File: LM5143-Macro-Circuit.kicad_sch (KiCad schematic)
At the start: 54 parts, among them Q2 NTMFS4D0N08XT1G, U10 NTMFS4D0N08XT1G, U11 NTMFS4D0N08XT1G, U14 NTMFS4D0N08XT1G, U15 NTMFS4D0N08XT1G, U8 LM5145

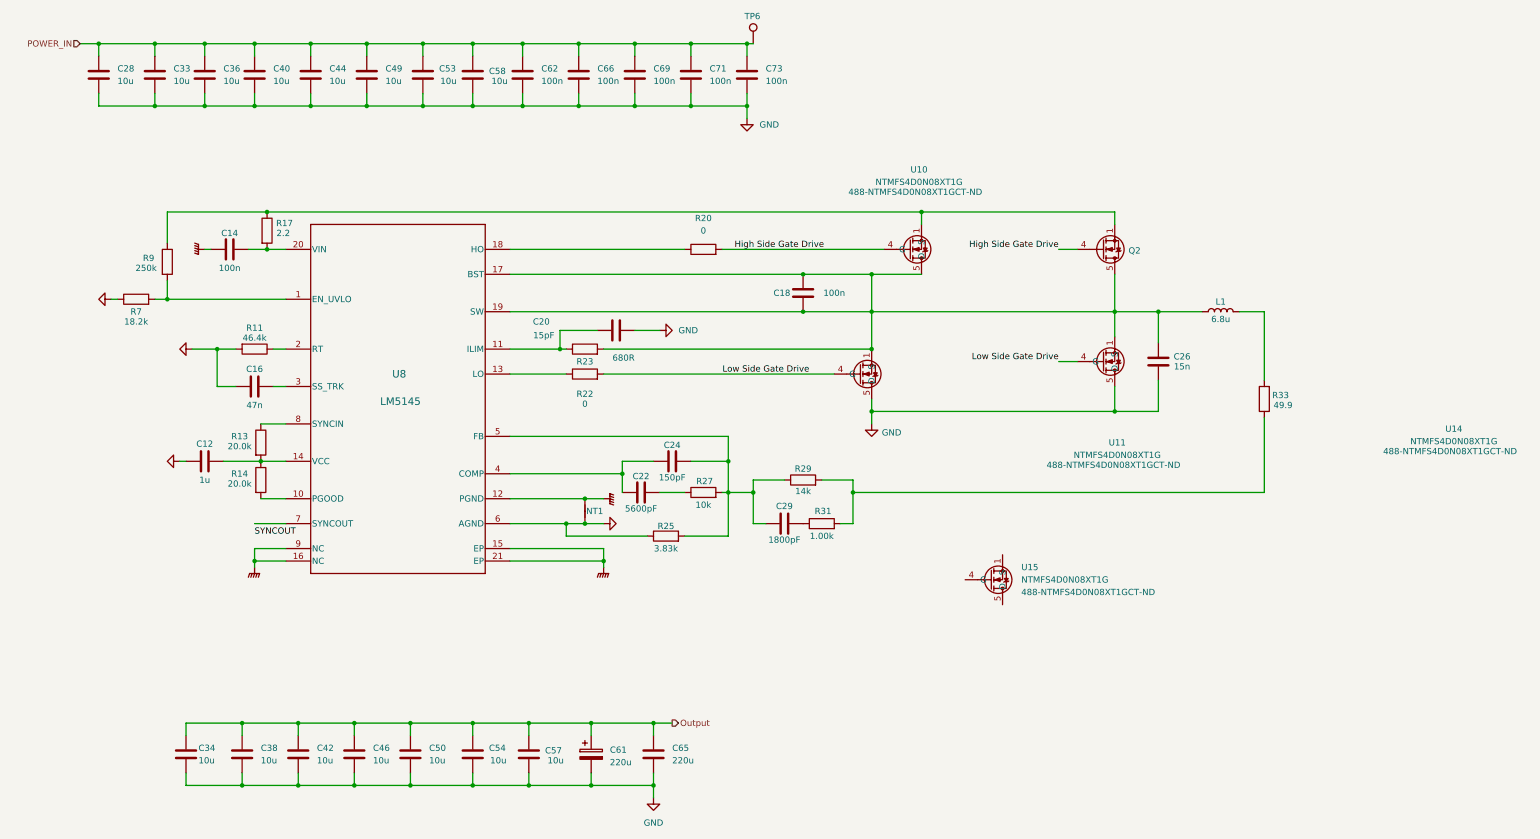
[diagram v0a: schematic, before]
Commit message: Started Layout and cleaned up schematic
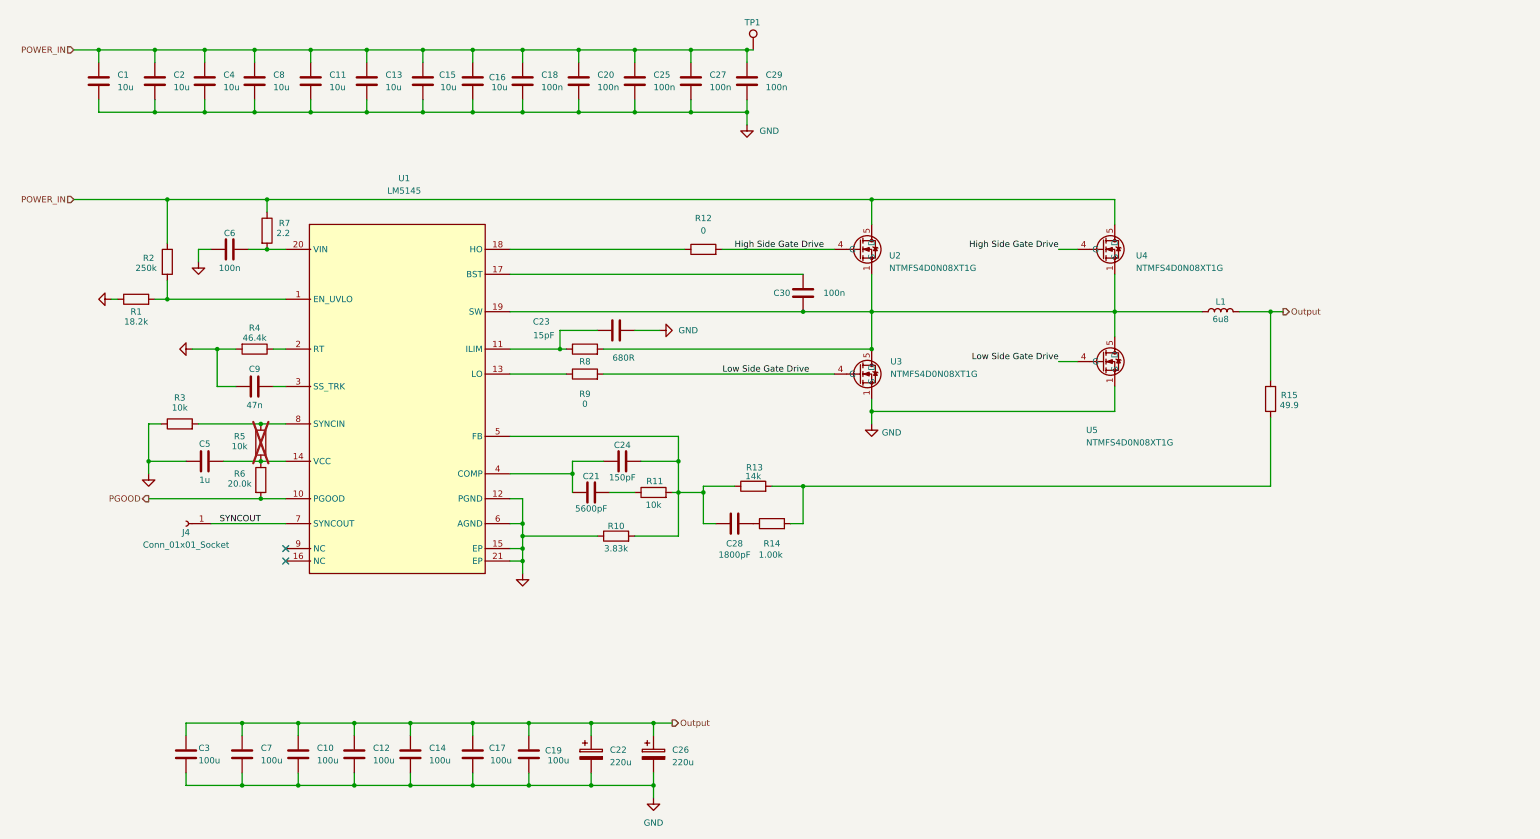
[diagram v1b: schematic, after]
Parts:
- removed C26: 15n, Capacitor_SMD:C_0603_1608Metric, symbol Device:C
- removed C65: 220u, Capacitor_SMD:C_0603_1608Metric, symbol Device:C
- removed NT1: NetTie_2, NetTie:NetTie-2_SMD_Pad0.5mm, symbol Device:NetTie_2
- removed Q2: NTMFS4D0N08XT1G, ecocad_lib_footprints:PowerMosDFNHybrid, symbol Transistor_FET:CSD18563Q5A
- removed U10, U11, U14, U15: NTMFS4D0N08XT1G, ecocad_lib_footprints:PowerMosDFNHybrid, symbol ecocad_lib_symbols:NTMFS4D0N08XT1G
- removed U8: LM5145, ecocad_lib_footprints:RGY0024F-MFG, symbol 2024-07-27_02-47-30:LM5145RGYR
- added C26: 220u, ecocad_lib_footprints:CAP_EEE1HA221P, symbol Device:C_Polarized
- added J4: Conn_01x01_Socket, Connector_PinHeader_2.54mm:PinHeader_1x01_P2.54mm_Vertical, symbol Connector:Conn_01x01_Socket
- added R3: 10k, Resistor_SMD:R_0603_1608Metric, symbol Device:R
- added U1: LM5145, Texas_RGY_R-PVQFN-N20_EP2.05x3.05mm_ThermalVias, symbol ecocad_lib_symbols:LM5145
- added U2, U3, U4, U5: NTMFS4D0N08XT1G, ecocad_lib_footprints:PowerMosDFNHybrid, symbol ecocad_lib_symbols:NTMFS4D0N08XT1G
- C10: renamed from C42; value 10u -> 100u
- C12: renamed from C46; value 10u -> 100u
- C14: renamed from C50; value 10u -> 100u
- C17: renamed from C54; value 10u -> 100u
- C19: renamed from C57; value 10u -> 100u
- C22: renamed from C61; footprint Capacitor_SMD:C_0603_1608Metric -> ecocad_lib_footprints:CAP_EEE1HA221P
- C3: renamed from C34; value 10u -> 100u
- C7: renamed from C38; value 10u -> 100u
- L1: value 6.8u -> 6u8
- R5: renamed from R13; value 20.0k -> 10k; now not fitted
- renumbered C28 to C1, C44 to C11, C49 to C13, C53 to C15, C58 to C16, C62 to C18, C33 to C2, C66 to C20, C22 to C21, C20 to C23, C69 to C25, C71 to C27, C29 to C28, C73 to C29, C18 to C30, C36 to C4, C12 to C5, C14 to C6, C40 to C8, C16 to C9, R7 to R1, R25 to R10, R27 to R11, R20 to R12, R29 to R13, R31 to R14, R33 to R15, R9 to R2, R11 to R4, R14 to R6, R17 to R7, R23 to R8, R22 to R9, TP6 to TP1
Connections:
- net GNDPWR is gone; now on net GND: C6.1
- net GND: now also C26.2, R3.1, U1.12 (PGND), U1.15 (EP), U1.21 (EP), U1.6 (AGND), U3.1 (S), U3.2 (S), U3.3 (S), U5.1 (S), U5.2 (S), U5.3 (S)
- net High Side Gate Drive: now also U2.4 (G), U4.4 (G)
- net Low Side Gate Drive: now also U3.4 (G), U5.4 (G)
- net Output: now also L1.2, R15.2, C26.1
- net POWER_IN: now also R2.1, R7.1, U2.5 (D), U4.5 (D)
- net SYNCOUT: now also J4.1 (Pin_1), U1.7 (SYNCOUT)
- net at C30.1, L1.1, R8.2: now also U1.19 (SW), U2.1 (S), U2.2 (S), U2.3 (S), U3.5 (D), U4.1 (S), U4.2 (S), U4.3 (S), U5.5 (D); no longer C30.2
- net at R5.1: now also R3.2, U1.8 (SYNCIN)
- net at C5.2, R5.2, R6.1: now also U1.14 (VCC)
- net at C24.2, C28.1, R10.2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: now also U1.5 (FB)
- net at C21.1, C24.1: now also U1.4 (COMP)
- net at R9.1: now also U1.13 (LO)
- net at R1.2, R2.2: now also U1.1 (EN_UVLO)
- net at R12.1: now also U1.18 (HO)
- net at C23.2, R8.1: now also U1.11 (ILIM)
- net PGOOD: now reaches R6.2
- net PGOOD: now also U1.10 (PGOOD)
- net at R4.1: now also U1.2 (RT)
- net at C6.2, R7.2: now also U1.20 (VIN)
- net at C9.2: now also U1.3 (SS_TRK)
- new net: C30.2, U1.17 (BST)
- no-connect marks 0 -> 2
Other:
- moved on the sheet: C1, C11, C13, C15, C16, C18, C2, C20, C21, C24, C25, C27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
